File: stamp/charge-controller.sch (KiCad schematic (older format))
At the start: 8 parts

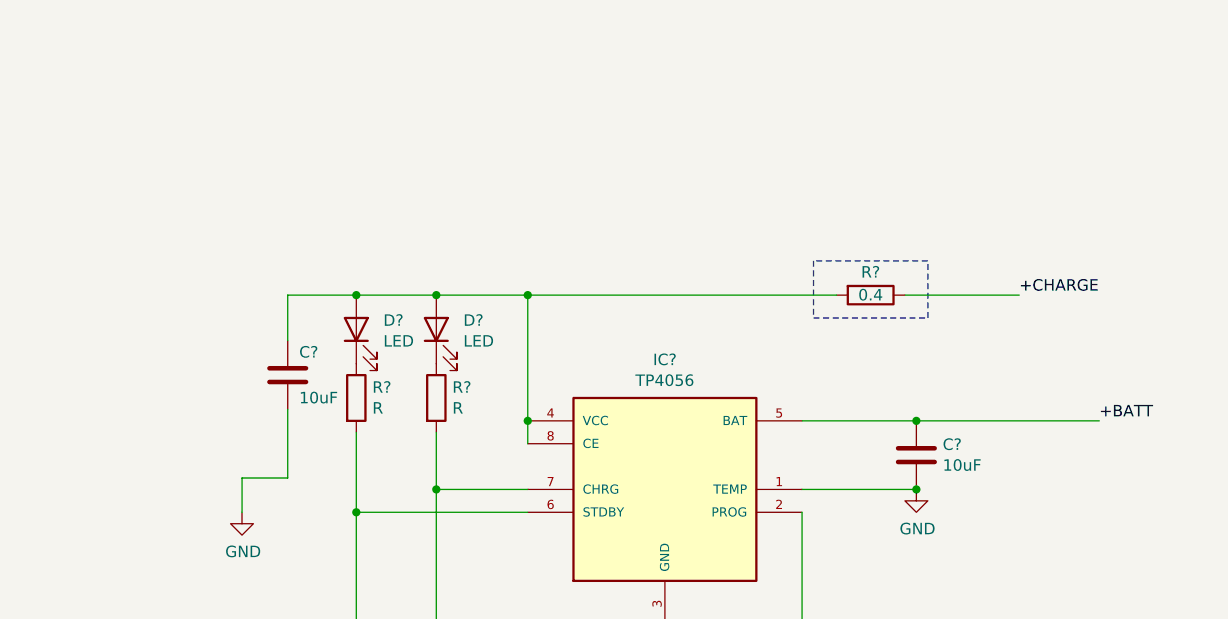
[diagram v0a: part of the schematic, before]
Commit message: Pre-review
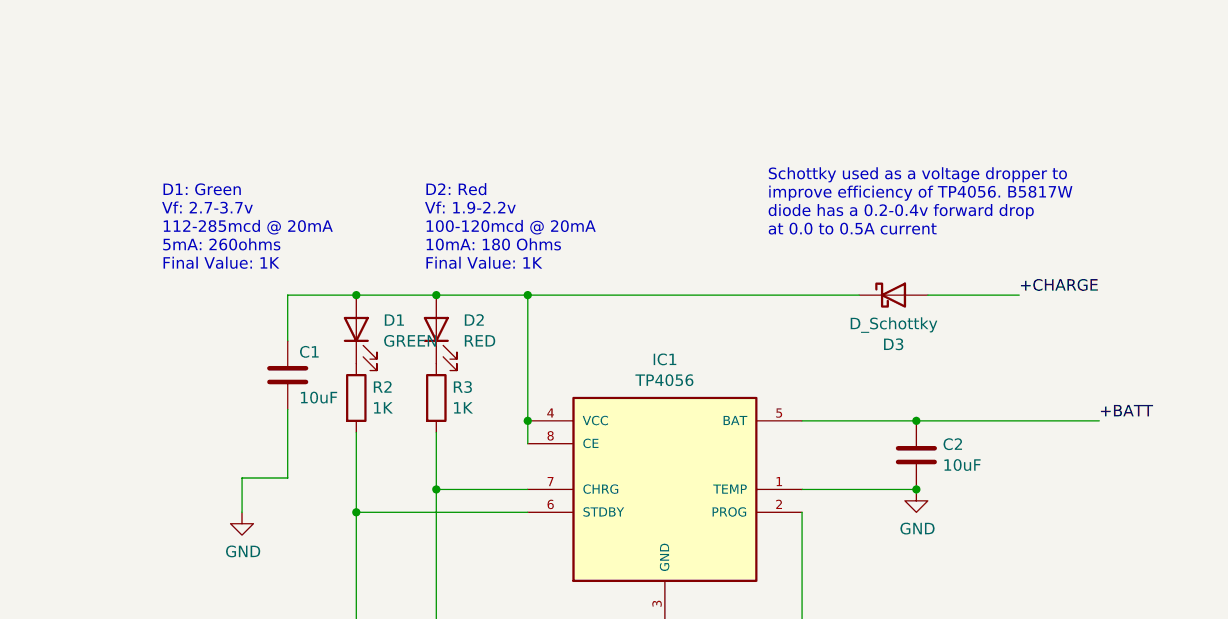
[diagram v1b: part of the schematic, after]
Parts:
- removed R?: 0.4, Resistor_SMD:R_0805_2012Metric, symbol Device:R
- added D3: D_Schottky, Diode_SMD:D_SOD-123, symbol Device:D_Schottky
- C1, C2: renamed from C?; footprint Capacitor_SMD:C_0402_1005Metric -> Capacitor_SMD:C_0805_2012Metric
- D1: renamed from D?; value LED -> GREEN
- D2: renamed from D?; value LED -> RED
- R2, R3: renamed from R?; value R -> 1K
- gave numbers to parts that had none: 1
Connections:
- net +CHARGE: now also D3.2 (A)
- net at C1.1, D1.2 (A), D2.2 (A)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: now also D3.1 (K)
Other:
- note added: "D1: Green\nVf: 2.7-3.7v\n112-285mcd @ 20mA\n5mA: 260ohms\nFinal Value: 1K"
- note added: "D2: Red\nVf: 1.9-2.2v\n100-120mcd @ 20mA\n10mA: 180 Ohms\nFinal Value: 1K"
- note added: "Schottky used as a voltage dropper to\nimprove efficiency of TP4056. B5817W\ndiode has a 0.2-0.4v forward drop\nat 0.0 to 0.5A current"
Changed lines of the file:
@@
 ~CHRG
 $Comp
-L Everything:TP4056 IC?
+L Everything:TP4056 IC1
 U 1 1 5FC5BC22
 P 5800 3100
-F 0 "IC?" H 5800 3667 50  0000 C CNN
+F 0 "IC1" H 5800 3667 50  0000 C CNN
 F 1 "TP4056" H 5800 3576 50  0000 C CNN
 F 2 "Everything:SOP-8" H 5800 3100 50  0001 L BNN
@@
 	1    0    0    -1
 $EndComp
-$Comp
-L Device:R R?
-U 1 1 5FC5BC28
-P 6700 2250
-F 0 "R?" V 6600 2250 50  0000 C CNN
-F 1 "0.4" V 6700 2250 50  0000 C CNN
-F 2 "Resistor_SMD:R_0805_2012Metric" V 6630 2250 50  0001 C CNN
-F 3 "~" H 6700 2250 50  0001 C CNN
-	1    6700 2250
-	0    1    1    0
-$EndComp
-Wire Notes Line
-	6450 2350 6950 2350
-Wire Notes Line
-	6950 2350 6950 2100
-Wire Notes Line
-	6950 2100 6450 2100
-Wire Notes Line
-	6450 2100 6450 2350
-Wire Wire Line
-	6550 2250 5200 2250
 Wire Wire Line
 	5200 2250 5200 2800
@@
 	5200 2800 5200 2900
 Connection ~ 5200 2800
-Connection ~ 5200 2250
-$Comp
-L power:GND #PWR?
+$Comp
+L power:GND #PWR0101
 U 1 1 5FC5BC37
 P 3950 3200
-F 0 "#PWR?" H 3950 2950 50  0001 C CNN
+F 0 "#PWR0101" H 3950 2950 50  0001 C CNN
 F 1 "GND" H 3955 3027 50  0000 C CNN
 F 2 "" H 3950 3200 50  0001 C CNN
@@
 	4150 2250 4450 2250
 $Comp
-L Device:R R?
+L Device:R R3
 U 1 1 5FC5BC3F
 P 4800 2700
-F 0 "R?" H 4870 2746 50  0000 L CNN
-F 1 "R" H 4870 2655 50  0000 L CNN
+F 0 "R3" H 4870 2746 50  0000 L CNN
+F 1 "1K" H 4870 2655 50  0000 L CNN
 F 2 "Resistor_SMD:R_0402_1005Metric" V 4730 2700 50  0001 C CNN
 F 3 "~" H 4800 2700 50  0001 C CNN
@@
 $EndComp
 $Comp
-L Device:R R?
+L Device:R R2
 U 1 1 5FC5BC45
 P 4450 2700
-F 0 "R?" H 4520 2746 50  0000 L CNN
-F 1 "R" H 4520 2655 50  0000 L CNN
+F 0 "R2" H 4520 2746 50  0000 L CNN
+F 1 "1K" H 4520 2655 50  0000 L CNN
 F 2 "Resistor_SMD:R_0402_1005Metric" V 4380 2700 50  0001 C CNN
 F 3 "~" H 4450 2700 50  0001 C CNN
@@
 $EndComp
 $Comp
-L Device:LED D?
+L Device:LED D1
 U 1 1 5FC5BC4B
 P 4450 2400
-F 0 "D?" V 4489 2282 50  0000 R CNN
-F 1 "LED" V 4398 2282 50  0000 R CNN
+F 0 "D1" V 4489 2282 50  0000 R CNN
+F 1 "GREEN" V 4398 2282 50  0000 R CNN
 F 2 "LED_SMD:LED_0603_1608Metric" H 4450 2400 50  0001 C CNN
 F 3 "~" H 4450 2400 50  0001 C CNN
@@
 $EndComp
 $Comp
-L Device:LED D?
+L Device:LED D2
 U 1 1 5FC5BC51
 P 4800 2400
-F 0 "D?" V 4839 2282 50  0000 R CNN
-F 1 "LED" V 4748 2282 50  0000 R CNN
+F 0 "D2" V 4839 2282 50  0000 R CNN
+F 1 "RED" V 4748 2282 50  0000 R CNN
 F 2 "LED_SMD:LED_0603_1608Metric" H 4800 2400 50  0001 C CNN
 F 3 "~" H 4800 2400 50  0001 C CNN
@@
 	4450 3200 5200 3200
 $Comp
-L power:GND #PWR?
+L power:GND #PWR0102
 U 1 1 5FC5BC5F
 P 5800 4400
-F 0 "#PWR?" H 5800 4150 50  0001 C CNN
+F 0 "#PWR0102" H 5800 4150 50  0001 C CNN
 F 1 "GND" H 5805 4227 50  0000 C CNN
 F 2 "" H 5800 4400 50  0001 C CNN
@@
 $EndComp
 $Comp
-L Device:C C?
+L Device:C C1
 U 1 1 5FC5BC65
 P 4150 2600
-F 0 "C?" H 4200 2700 50  0000 L CNN
+F 0 "C1" H 4200 2700 50  0000 L CNN
 F 1 "10uF" H 4200 2500 50  0000 L CNN
-F 2 "Capacitor_SMD:C_0402_1005Metric" H 4188 2450 50  0001 C CNN
+F 2 "Capacitor_SMD:C_0805_2012Metric" H 4188 2450 50  0001 C CNN
 F 3 "~" H 4150 2600 50  0001 C CNN
 	1    4150 2600
@@
 $EndComp
 $Comp
-L Device:C C?
+L Device:C C2
 U 1 1 5FC5BC6C
 P 6900 2950
-F 0 "C?" H 7015 2996 50  0000 L CNN
+F 0 "C2" H 7015 2996 50  0000 L CNN
 F 1 "10uF" H 7015 2905 50  0000 L CNN
-F 2 "Capacitor_SMD:C_0402_1005Metric" H 6938 2800 50  0001 C CNN
+F 2 "Capacitor_SMD:C_0805_2012Metric" H 6938 2800 50  0001 C CNN
 F 3 "~" H 6900 2950 50  0001 C CNN
 	1    6900 2950
@@
 Connection ~ 6900 2800
 $Comp
-L power:GND #PWR?
+L power:GND #PWR0103
 U 1 1 5FC5BC74
 P 6900 3100
-F 0 "#PWR?" H 6900 2850 50  0001 C CNN
+F 0 "#PWR0103" H 6900 2850 50  0001 C CNN
 F 1 "GND" H 6905 2927 50  0000 C CNN
 F 2 "" H 6900 3100 50  0001 C CNN
@@
 Wire Wire Line
 	6400 3100 6900 3100
-Wire Wire Line
-	6850 2250 7350 2250
 Wire Wire Line
 	6900 2800 7700 2800
@@
 PROG
 $Comp
-L power:GND #PWR?
+L power:GND #PWR0104
 U 1 1 5FC63996
 P 1450 1500
-F 0 "#PWR?" H 1450 1250 50  0001 C CNN
+F 0 "#PWR0104" H 1450 1250 50  0001 C CNN
 F 1 "GND" H 1455 1327 50  0000 C CNN
 F 2 "" H 1450 1500 50  0001 C CNN
@@
 Wire Wire Line
 	6400 3800 6850 3800
+$Comp
+L Device:D_Schottky D?
+U 1 1 5FC3EFB8
+P 6800 2250
+AR Path="/5FC721ED/5FC3EFB8" Ref="D?"  Part="1"
+AR Path="/5FC467D5/5FC3EFB8" Ref="D3"  Part="1"
+F 0 "D3" H 6800 2033 50  0000 C CNN
+F 1 "D_Schottky" H 6800 2124 50  0000 C CNN
+F 2 "Diode_SMD:D_SOD-123" H 6800 2250 50  0001 C CNN
+F 3 "~" H 6800 2250 50  0001 C CNN
+	1    6800 2250
+	1    0    0    -1
+$EndComp
+Wire Wire Line
+	7350 2250 6950 2250
+Wire Wire Line
+	6650 2250 5200 2250
+Connection ~ 5200 2250
+Text Notes 6250 2000 0    50   ~ 0
+Schottky used as a voltage dropper to\nimprove efficiency of TP4056. B5817W\ndiode has a 0.2-0.4v forward drop\nat 0.0 to 0.5A current
+Text Notes 3600 2150 0    50   ~ 0
+D1: Green\nVf: 2.7-3.7v\n112-285mcd @ 20mA\n5mA: 260ohms\nFinal Value: 1K
+Text Notes 4750 2150 0    50   ~ 0
+D2: Red\nVf: 1.9-2.2v\n100-120mcd @ 20mA\n10mA: 180 Ohms\nFinal Value: 1K
 $EndSCHEMATC
